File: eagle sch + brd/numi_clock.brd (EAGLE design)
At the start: 71.2 x 30.1 mm, 30 parts, among them IC1 MEGA8-AI, IC2 LM75, Q1 12MHz, Y1 32.768kHz

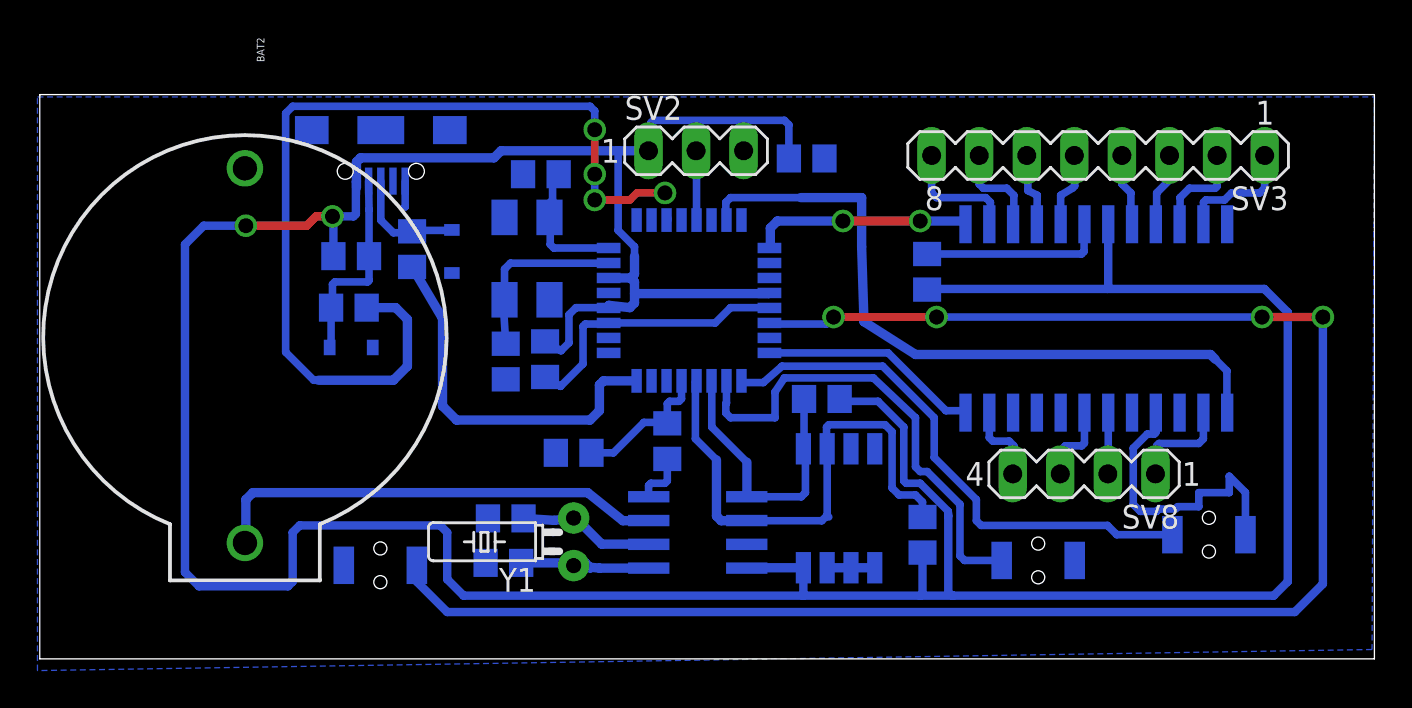
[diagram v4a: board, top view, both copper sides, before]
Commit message: routed all tracks
routed all tracks
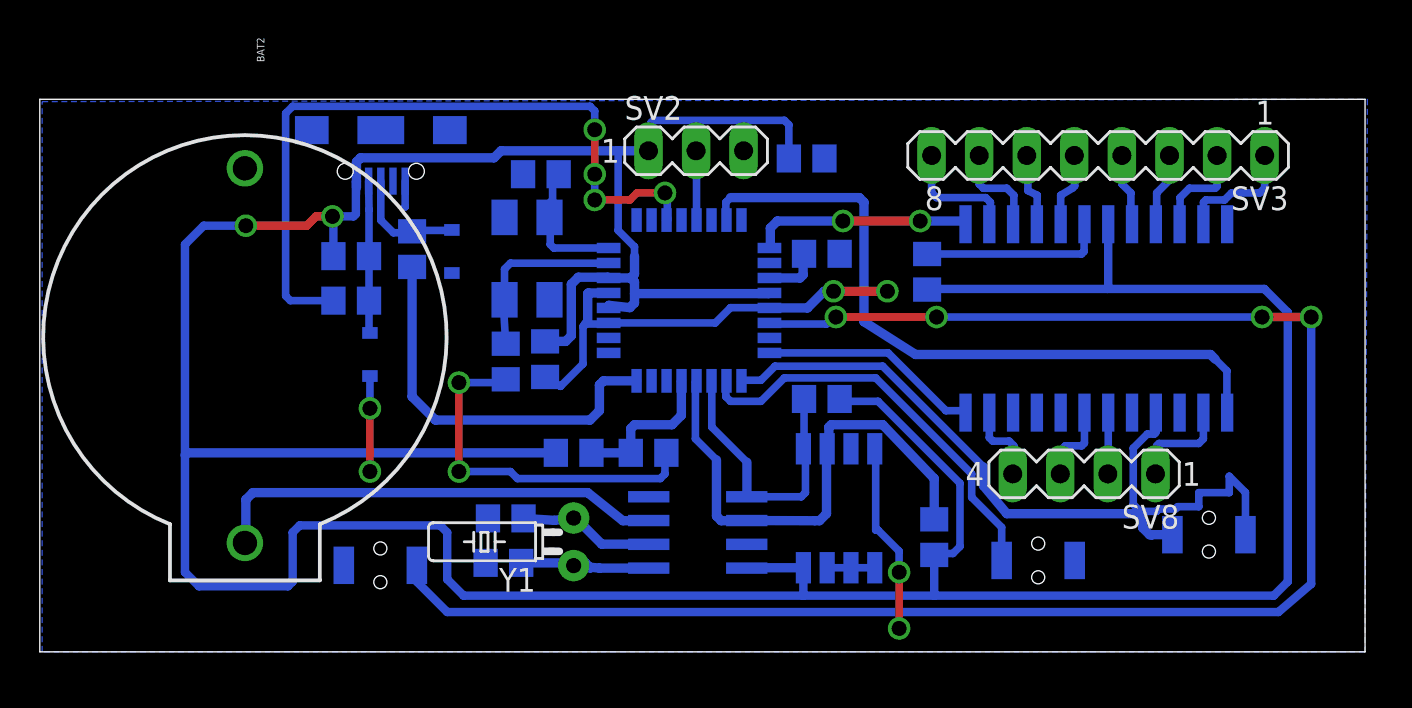
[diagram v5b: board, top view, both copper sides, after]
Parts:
- added D3: (no value), sym:R0805
- moved C1 1.18 mm to (47.6, 18.6), turned to 0 degrees
- moved D1 1.07 mm to (32.8, 23.9), turned to 270 degrees
- moved R10 0.64 mm to (62.9, 14.1)
- moved R2 0.40 mm to (31.8, 26.8), turned to 0 degrees
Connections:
- new net LED: D3.1, IC1.19
- net GND: now also D3.2
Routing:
- net GND: track 38.7 -> 80.4 mm, vias 0 -> 8
- net +5V: track 208.1 -> 227.3 mm
- net N$10: track 50.6 -> 39.3 mm
- net HOUR: track 25.5 -> 22.0 mm
- net LED: track 0.00 -> 3.01 mm
- net N$8: track 10.8 -> 8.16 mm
- net FUNC: track 94.5 -> 93.2 mm
- net MINUTE: track 29.0 -> 28.0 mm
- net N$9: track 20.2 -> 21.1 mm
- net RESET: track 7.62 -> 8.24 mm
- net SCL: track 28.1 -> 27.6 mm
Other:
- board size 71.2 x 30.1 mm -> 70.8 x 29.5 mm
